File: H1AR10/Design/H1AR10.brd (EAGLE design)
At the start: 34.6 x 30 mm, 42 parts, among them P1 HEXABIT_17.32_NO_P3, U1 STM32F091CBU6, U2 FT230XQ, U3 TI_NATIONAL_SEMICONDUCTOR_LM3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, X1 XTALL_CSTCE8M00G52, X3 USB-B-H

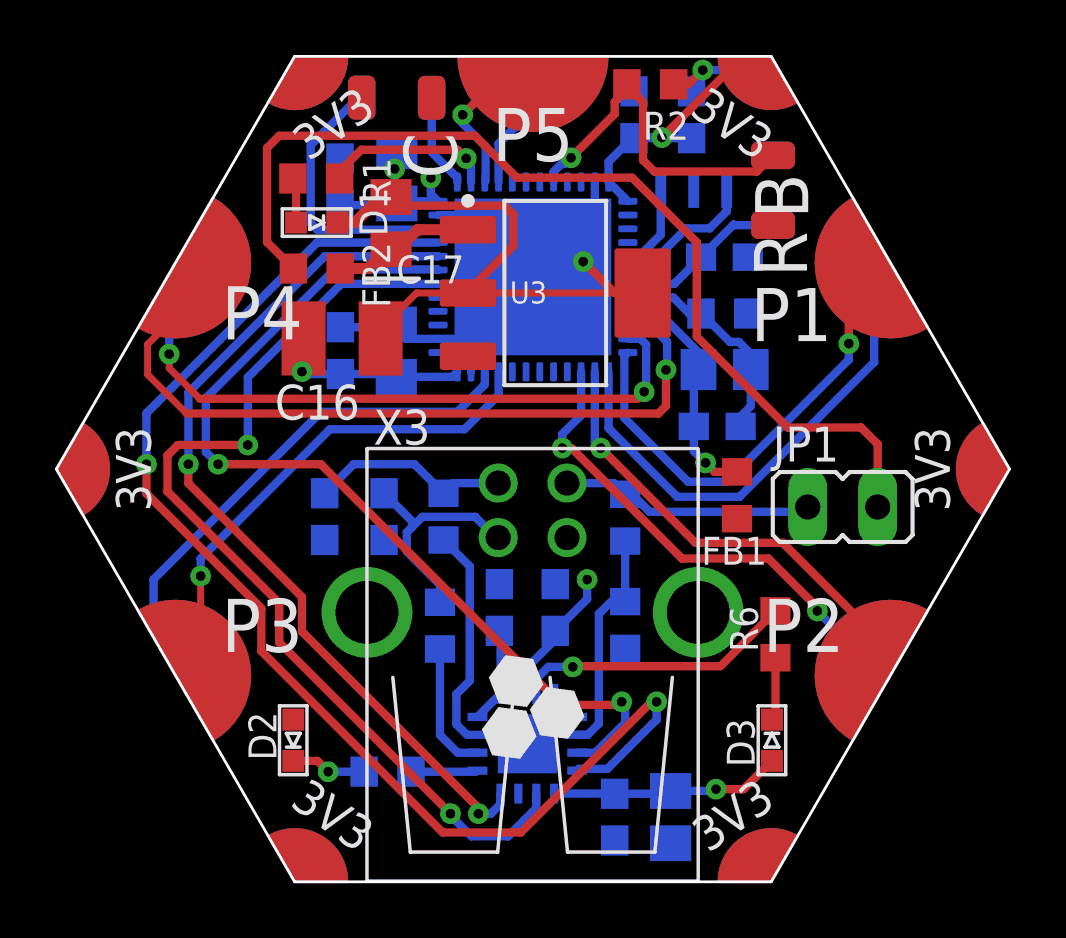
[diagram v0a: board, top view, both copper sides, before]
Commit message: final un-checked
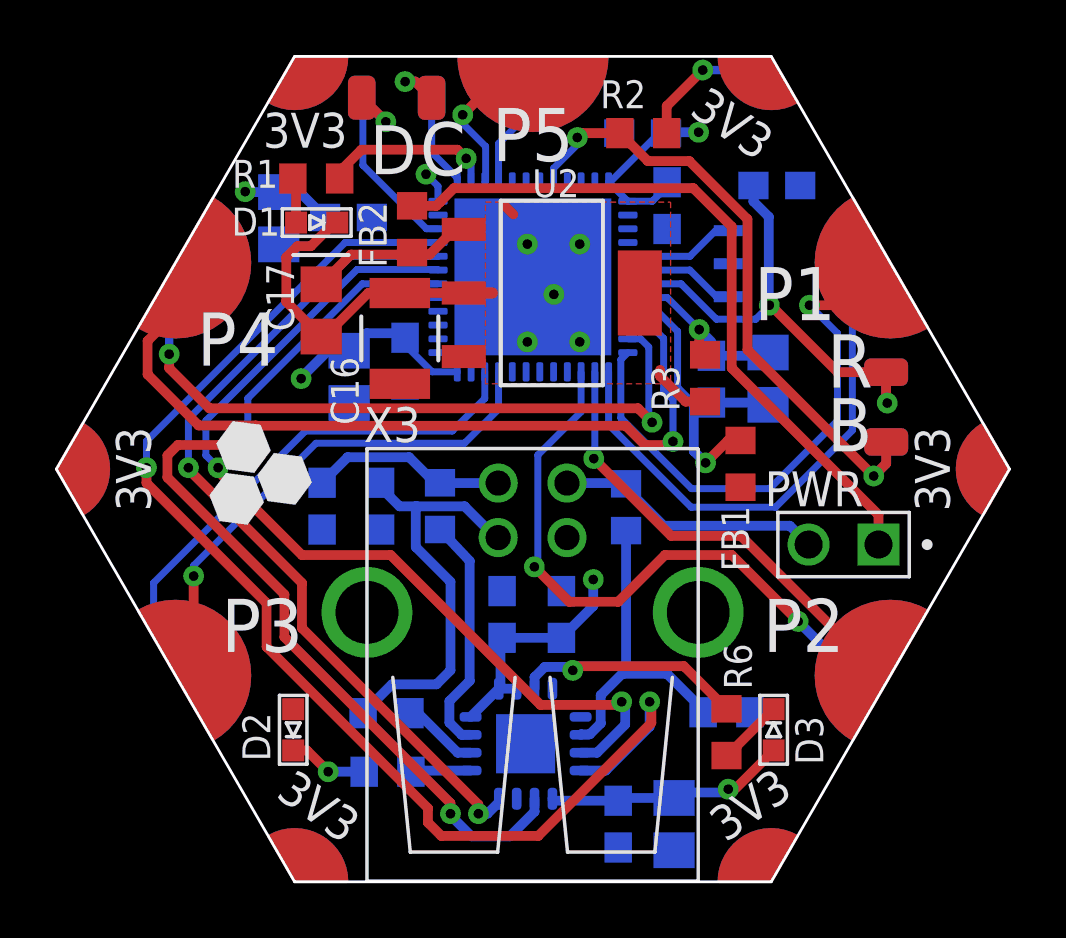
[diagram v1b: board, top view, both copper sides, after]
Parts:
- removed JP1: (no value), Hexabitz:JP1
- removed U3: TI_NATIONAL_SEMICONDUCTOR_LM3940IMP-3.3TI_NATIONAL_SEMICOND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, TI National Semiconductor - LM3940IMP-3.3:TI_NATIONAL_SEMICONDUCTOR_LM3940IMP-3.3_2
- added PWR: 3-644456-2, Hexabitz:TE_3-644456-2
- added U4: FT230XQ-R, Hexabitz:QFN16
- C16: device Hexabitz:C3225 -> Hexabitz:C-3225
- D1, D2, D3: value VLMS1300-GS08 -> RED
- U2: value FT230XQ -> LM3940IMP-3.3; device Hexabitz:QFN16 -> Hexabitz:SOT230P696X180-4N
- moved U2 16.4 mm to (35.3, 41.0), flipped to the top, turned to 0 degrees
- moved B 11.2 mm to (47.5, 35.6), turned to 180 degrees
- moved R 6.74 mm to (47.5, 38.1), turned to 180 degrees
- moved R9 4.86 mm to (41.7, 25.8), turned to 0 degrees
- moved C3 4.54 mm to (25.4, 43.7), turned to 270 degrees
- moved C17 4.07 mm to (26.9, 40.4), turned to 270 degrees
- moved R6 3.98 mm to (41.7, 25.1)
- moved FB2 3.74 mm to (30.2, 43.3), turned to 270 degrees
- moved R5 3.73 mm to (29.3, 25.7), turned to 0 degrees
- moved C7 3.42 mm to (39.5, 44.2), turned to 270 degrees
- moved C1 3.23 mm to (43.5, 44.9)
- moved X1 3.08 mm to (41.9, 42.1), turned to 0 degrees
- moved R3 2.45 mm to (40.9, 37.9), flipped to the top, turned to 90 degrees
- moved C8 2.38 mm to (30.0, 38.5), turned to 270 degrees
- moved C16 2.10 mm to (29.8, 39.4), turned to 90 degrees
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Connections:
- removed net VDD2: C15.1, U2.8, U2.9
- net GND: now also U1.P$2, U2.2, U2.4, U4.13, U4.17, U4.3; no longer U1.P$26, U1.P$43, U2.13, U2.3, U2.EXP, U3.2, U3.4
- net N$10: now also U4.11; no longer U2.11
- net N$11: now also U4.7; no longer U2.7
- net N$12: now also U4.6; no longer U2.6
- net N$15: now also PWR.1; no longer JP1.2
- net N$16: now also U2.1; no longer U3.1
- net N$17: now also PWR.2; no longer JP1.1
- net N$3: now also U4.5; no longer U2.5
- net UART1_CTS: now also U4.4; no longer U2.4
- net UART1_RTS: now also U4.16; no longer U2.16
- net UART1_RX: now also U4.15; no longer U2.15
- net UART1_TX: now also U4.2; no longer U2.2
- net VBUS_SENSE: now also U4.14; no longer U2.14
- net VDD: now also C15.1, U2.3, U4.1, U4.10, U4.8, U4.9; no longer U2.1, U2.10, U3.3
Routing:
- net GND: track 38.0 -> 20.4 mm, vias 3 -> 6
- net R1: track 6.22 -> 18.0 mm, vias 0 -> 2
- net B1: track 13.1 -> 23.6 mm, vias 1 -> 2
- net N$15: track 36.1 -> 26.2 mm
- net N$13: track 8.56 -> 15.5 mm
- net UART6_RX: track 17.7 -> 23.0 mm
- net VBUS_SENSE: track 8.28 -> 11.9 mm
- net VDD2: track 3.48 -> 0.00 mm
- net UART2_TX: track 17.0 -> 19.9 mm
- net VDDA: track 8.91 -> 11.7 mm
- net VDD: track 34.6 -> 37.4 mm, vias 5 -> 6
- net N$9: track 3.45 -> 5.86 mm, vias 0 -> 1
- net UART4_TX: track 28.0 -> 30.0 mm
- net N$10: track 10.3 -> 8.31 mm
- net N$12: track 4.75 -> 2.80 mm
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- added copper zone on layer 1, net GND
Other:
- board text added: "D"
